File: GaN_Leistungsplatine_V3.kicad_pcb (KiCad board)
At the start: 4 copper layers, 100 x 100 mm, 91 parts, among them J1 GPI0_1, J10 Conn_02x02_Top_Bottom, J2 105-1102-001, J3 105-1102-001, J4 105-1102-001, J5 105-1102-001, J6 105-1102-001, J7 105-1102-001, J8 105-1102-001, J9 Conn_02x03_Counter_Clockwise, Q1 GaN_FET_with_Source_Kelvin_Pin, Q2 GaN_FET_with_Source_Kelvin_Pin, U1 LT1999, U2 NCP51810

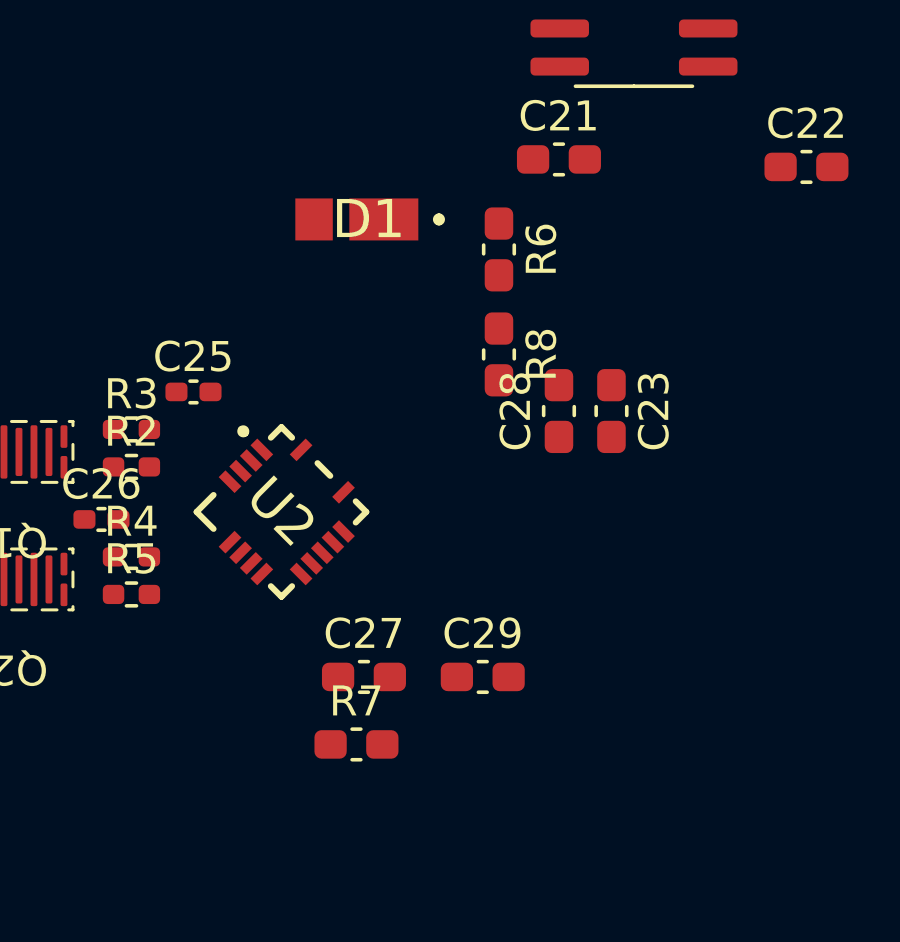
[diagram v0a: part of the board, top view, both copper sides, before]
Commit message: hello
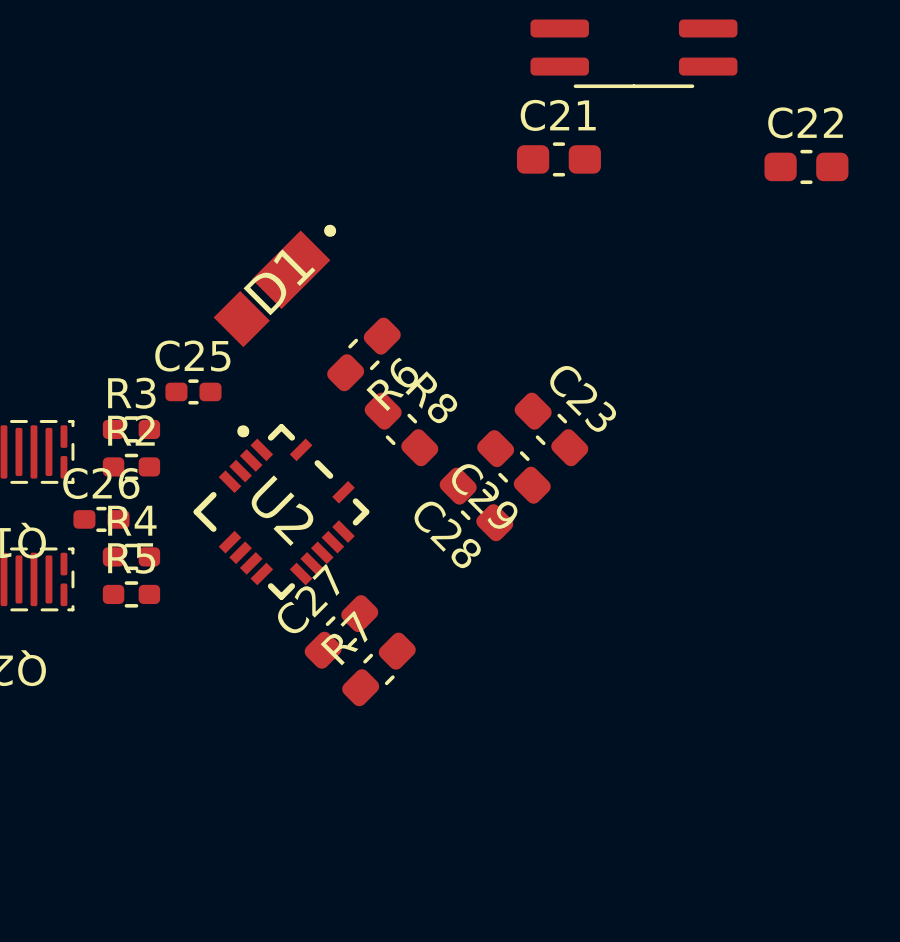
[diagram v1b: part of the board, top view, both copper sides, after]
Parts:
- moved C29 7.08 mm to (79.9, 106.2), turned to 135 degrees
- moved R6 5.70 mm to (74.9, 102.5), turned to -135 degrees
- moved C28 4.15 mm to (78.6, 107.5), turned to 135 degrees
- moved R8 4.10 mm to (76.1, 105.0), turned to -45 degrees
- moved D1 3.72 mm to (71.6, 100.5), turned to -135 degrees
- moved R7 2.61 mm to (75.4, 113.0), turned to 45 degrees
- moved C23 2.09 mm to (81.1, 105.0), turned to -45 degrees
- moved C27 1.68 mm to (74.1, 111.7), turned to 45 degrees
